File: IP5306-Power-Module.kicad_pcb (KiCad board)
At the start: 2 copper layers, 25 parts, among them J1 USB_C_Receptacle_USB2.0_16P, J2 S2B-XH-A_LF__SN_, J3 USB_A, J4 USB_A, SW1 KEY, U1 IP5306

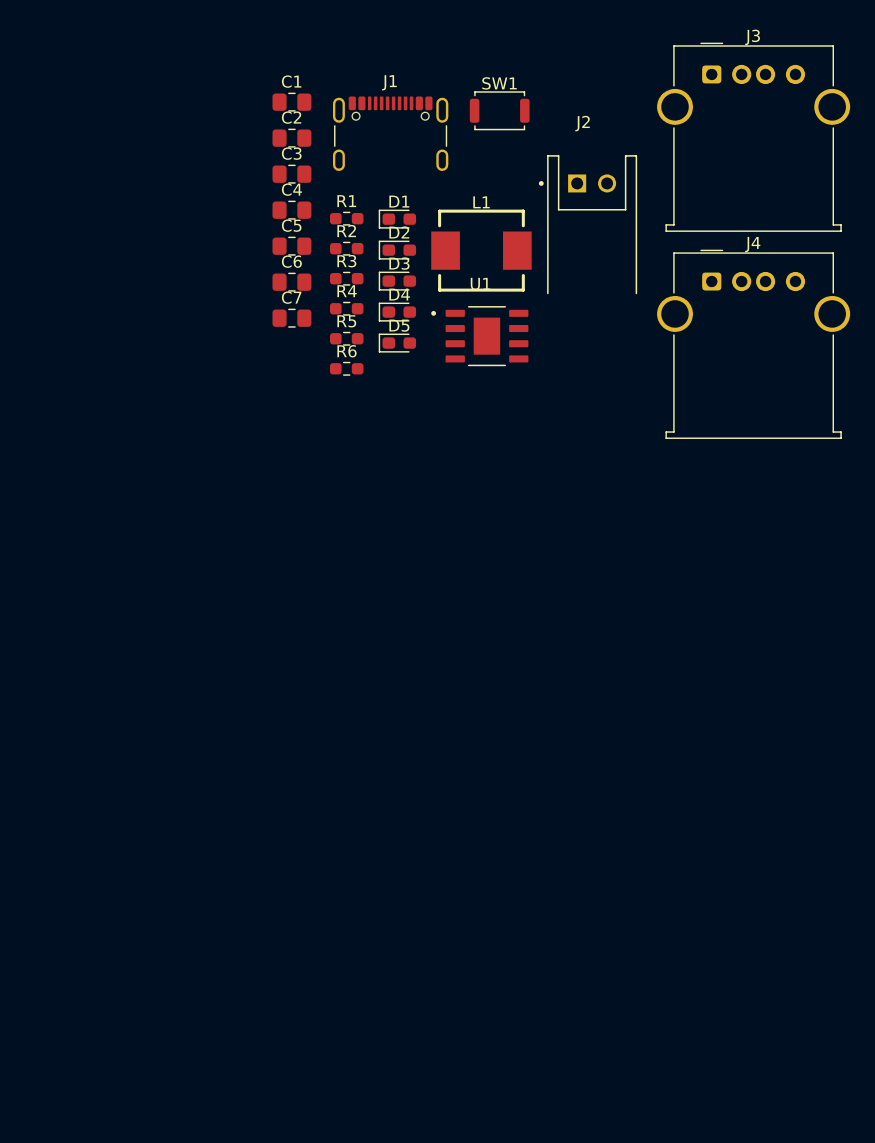
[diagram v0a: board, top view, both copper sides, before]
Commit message: V1
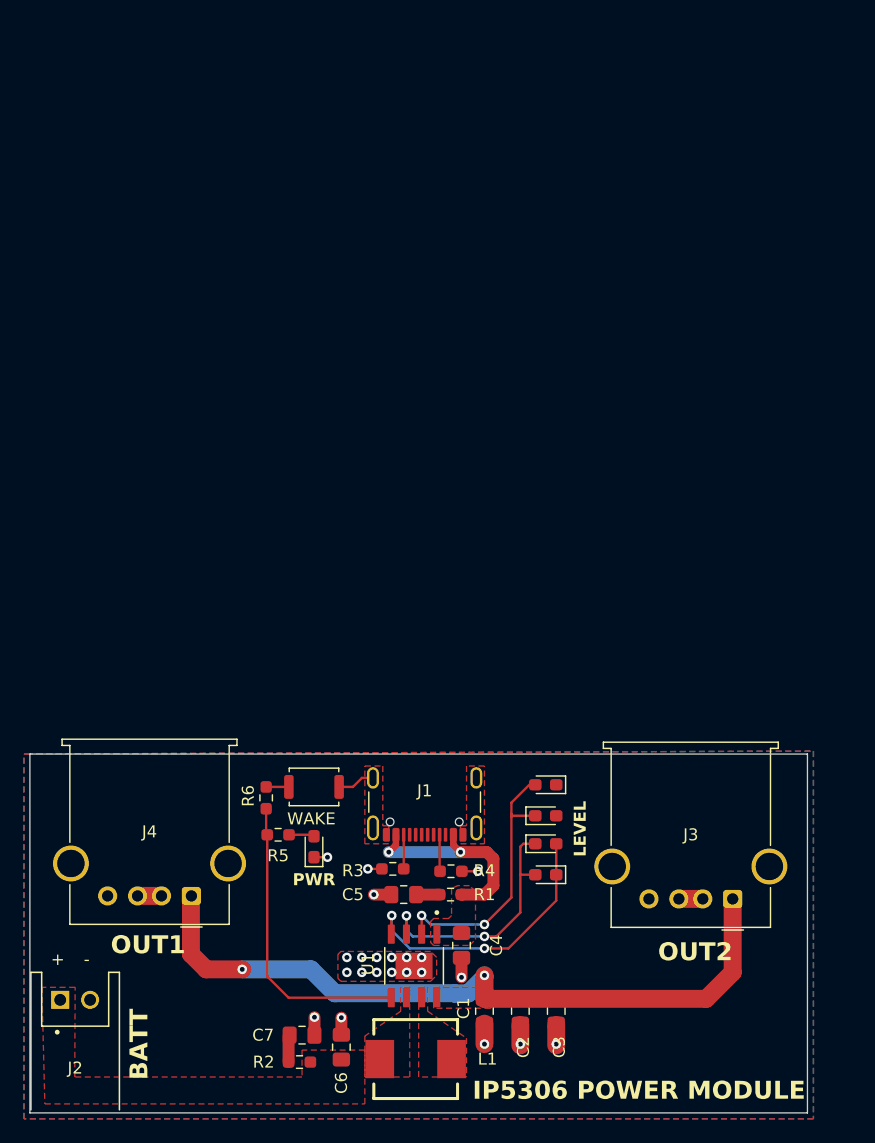
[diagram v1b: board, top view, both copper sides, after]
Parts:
- moved J2 80.8 mm to (123.8, 126.2)
- moved C1 77.7 mm to (158.0, 121.5), turned to -90 degrees
- moved C2 75.4 mm to (161.0, 121.5), turned to -90 degrees
- moved C3 73.4 mm to (164.0, 121.5), turned to -90 degrees
- moved J3 68.9 mm to (178.8, 112.1), turned to 180 degrees
- moved R2 68.1 mm to (142.5, 125.8), turned to 180 degrees
- moved L1 67.8 mm to (152.2, 125.5), turned to 180 degrees
- moved J4 67.3 mm to (133.5, 111.9), turned to 180 degrees
- moved C6 64.1 mm to (146.0, 124.5), turned to 90 degrees
- moved C4 63.1 mm to (156.1, 116.0), turned to -90 degrees
- moved C7 59.9 mm to (142.8, 123.5)
- moved LEVEL 58.6 mm to (143.8, 102.8)
- moved R1 57.2 mm to (155.2, 111.8), turned to 180 degrees
- moved C5 55.0 mm to (151.2, 111.8), turned to 180 degrees
- moved J1 53.9 mm to (153.0, 103.1), turned to 180 degrees
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- renumbered D3 to 100%, D1 to 25%, D2 to 50%, D4 to 75%, SW1 to LEVEL, D5 to PWR
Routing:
- net /VOUT: track 0.00 -> 61.3 mm, vias 0 -> 2
- net /KEY: track 0.00 -> 25.0 mm
- net /LED3: track 0.00 -> 23.6 mm, vias 0 -> 2
- net /LED1: track 0.00 -> 22.4 mm, vias 0 -> 2
- net /LED2: track 0.00 -> 21.4 mm, vias 0 -> 2
- net GND: track 0.00 -> 17.9 mm, vias 0 -> 22
- net /VIN: track 0.00 -> 17.6 mm, vias 0 -> 2
- net /CC1: track 0.00 -> 3.01 mm
- net /CC2: track 0.00 -> 2.85 mm
- net Net-(C7-Pad1): track 0.00 -> 2.16 mm
- net Net-(J4-D+): track 0.00 -> 2.00 mm
- net Net-(J3-D+): track 0.00 -> 2.00 mm
- net Net-(D5-A): track 0.00 -> 1.96 mm
- net Net-(C5-Pad1): track 0.00 -> 1.96 mm
- net Net-(R6-Pad2): track 0.00 -> 1.90 mm
- added copper zone on F.Cu, net /BAT
- added copper zone on F.Cu, net /SW
- added copper zone on F.Cu, net /VIN
- added copper zone on F.Cu, net /VOUT
- added copper zone on B.Cu, net GND
- added copper zone on F.Cu, net GND
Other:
- board outline added: 65 x 30 mm
- board text added: "+"
- board text added: "-"
- board text added: "BATT"
- board text added: "IP5306 POWER MODULE"
- board text added: "OUT1"
- board text added: "OUT2"
- board text added: "WAKE"
